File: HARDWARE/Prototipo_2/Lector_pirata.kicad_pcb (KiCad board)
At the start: 2 copper layers, 115 x 100 mm, 98 parts, among them J1 CONN_01X02, J10 PIN_3, J11 RJ45, J12 PIN_3, J13 PIN_3, J14 RJ45, J15 RJ45, J16 RJ45, J17 RJ45, J18 RJ45, J2 test Poins, J20 RJ45, J21 RJ45, J22 RJ45, J23 RJ45, J25 RJ45, J26 QR_1, J27 QR_2, J28 CONN_01X03, J29 CONN_01X03, J3 RESET, J4 CONN_01X06, J5 CONN_01X07, J6 CONN_01X05, J7 CONN_01X03, J8 CONN_01X03, J9 PIN_3, U1 TPS5622, U10 Max232, U11 Max232, U3 TM4C1231H6PM, U4 74HC125, U5 74HC125, U6 74HC125, U7 74HC125, U8 Microreader, U9 Microreader, Y1 16MHz, Y2 Crystal

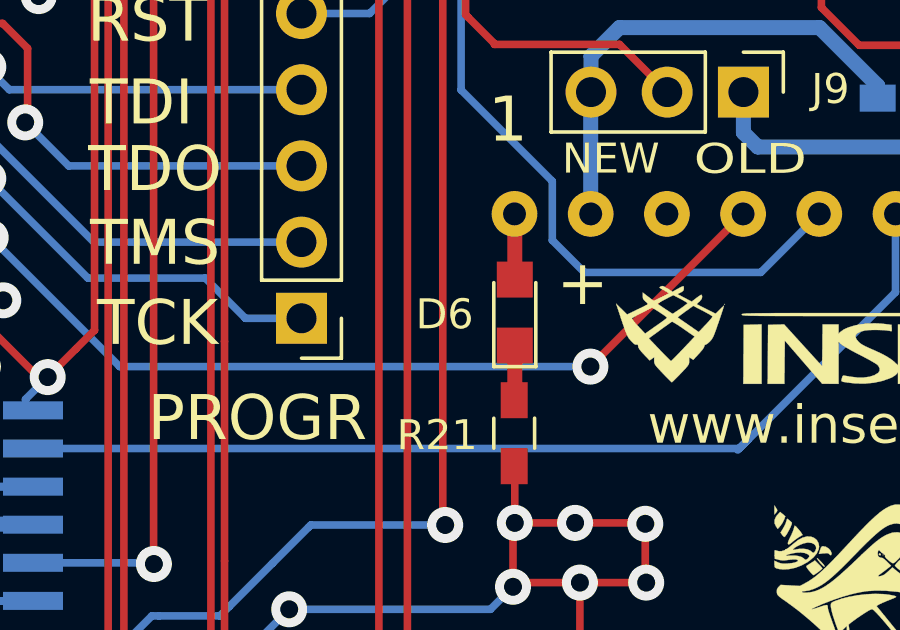
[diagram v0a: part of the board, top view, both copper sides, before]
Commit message: version_4
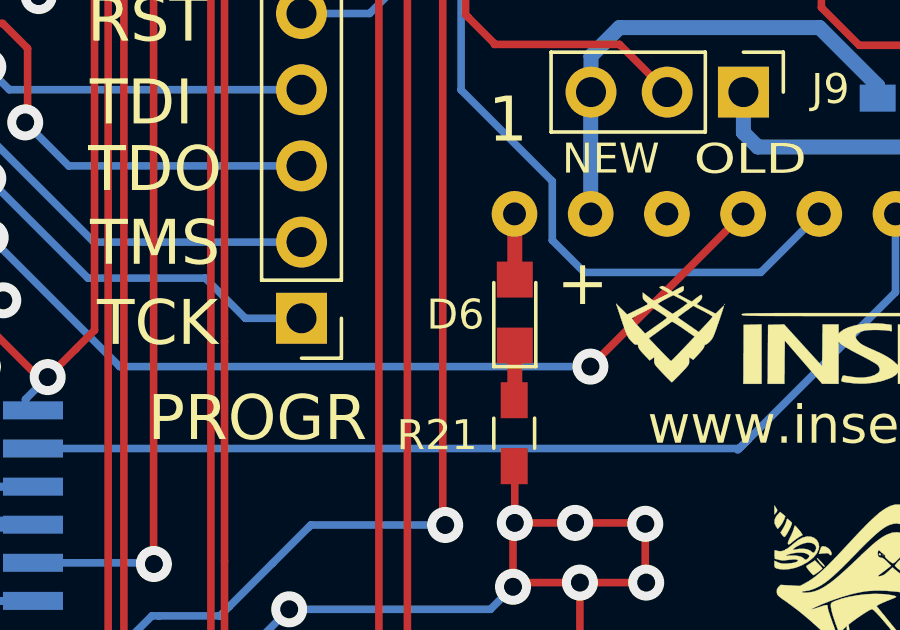
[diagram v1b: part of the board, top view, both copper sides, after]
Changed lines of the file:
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@@
   (page A4)
   (layers
-    (0 F.Cu signal hide)
+    (0 F.Cu signal)
     (31 B.Cu signal)
     (32 B.Adhes user hide)
@@
     (35 F.Paste user hide)
     (36 B.SilkS user)
-    (37 F.SilkS user hide)
+    (37 F.SilkS user)
     (38 B.Mask user)
     (39 F.Mask user)
@@
     (tags "LED led 0805 SMD smd SMT smt smdled SMDLED smtled SMTLED")
     (attr smd)
-    (fp_text reference D6 (at -0.06 -2.34 180) (layer F.SilkS)
+    (fp_text reference D6 (at -0.07 -1.98 180) (layer F.SilkS)
       (effects (font (size 1 1) (thickness 0.15)))
     )
